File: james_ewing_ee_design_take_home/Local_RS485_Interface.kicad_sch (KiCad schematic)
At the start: 45 parts, among them J1 USB_B_Micro, J3 RJ45, J5 Conn_Coaxial, SW1 RST, SW2 RST, SW3 RST, U1 ESP8266EX, U1 SN65176BDR, U2 MCP2200-E-SS, U5 M95M02-DR, Y1 Resonator, Y2 TSX-3225

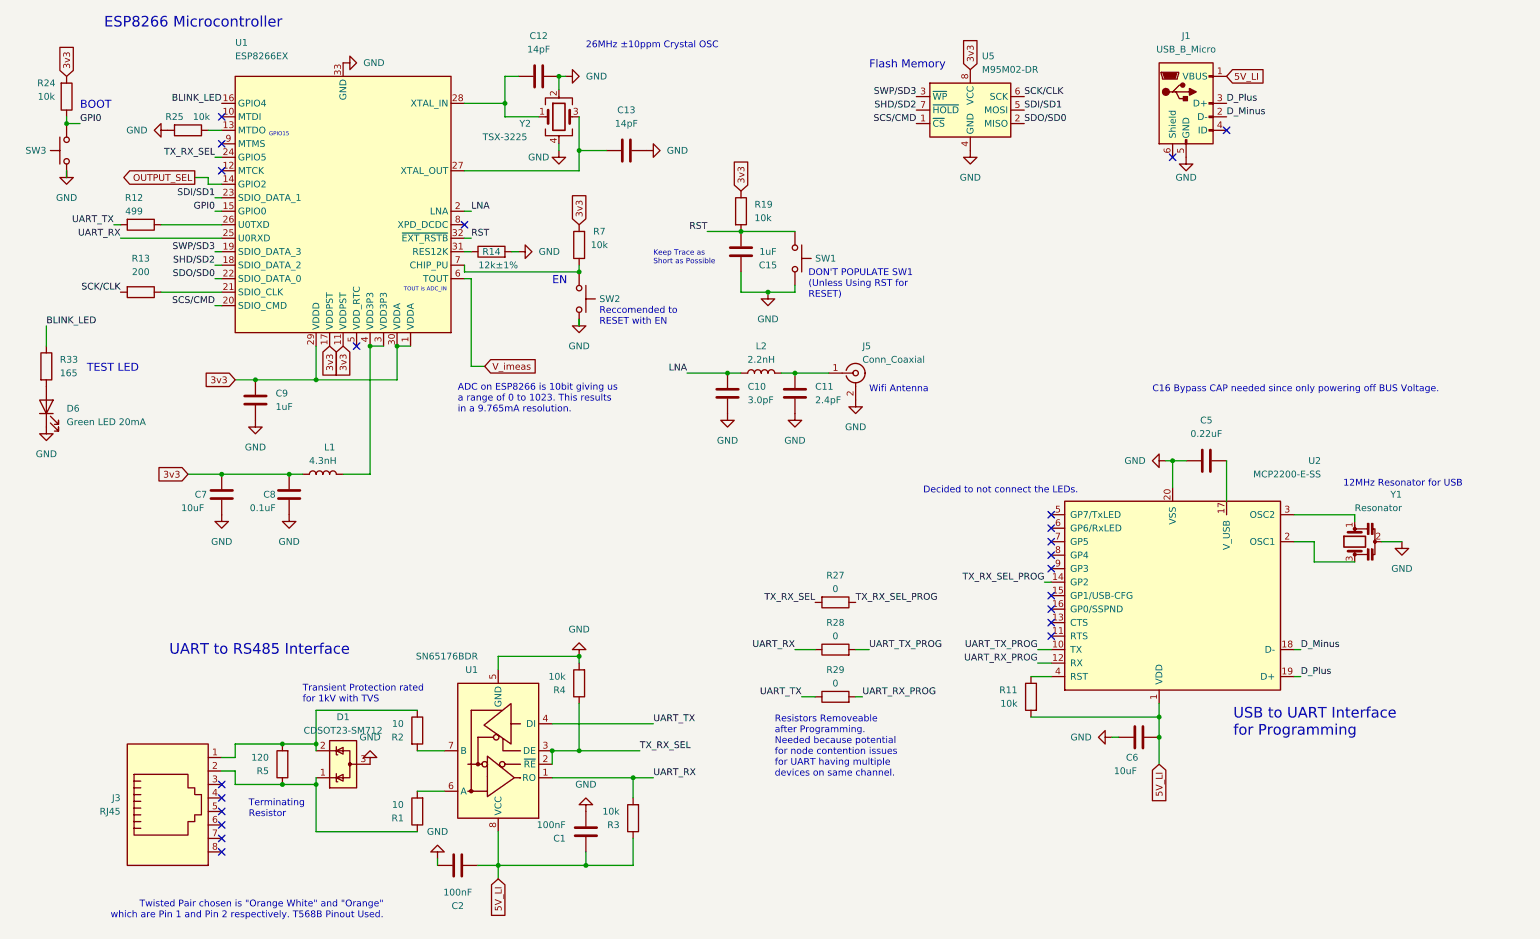
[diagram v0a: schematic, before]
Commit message: Updated Documentation
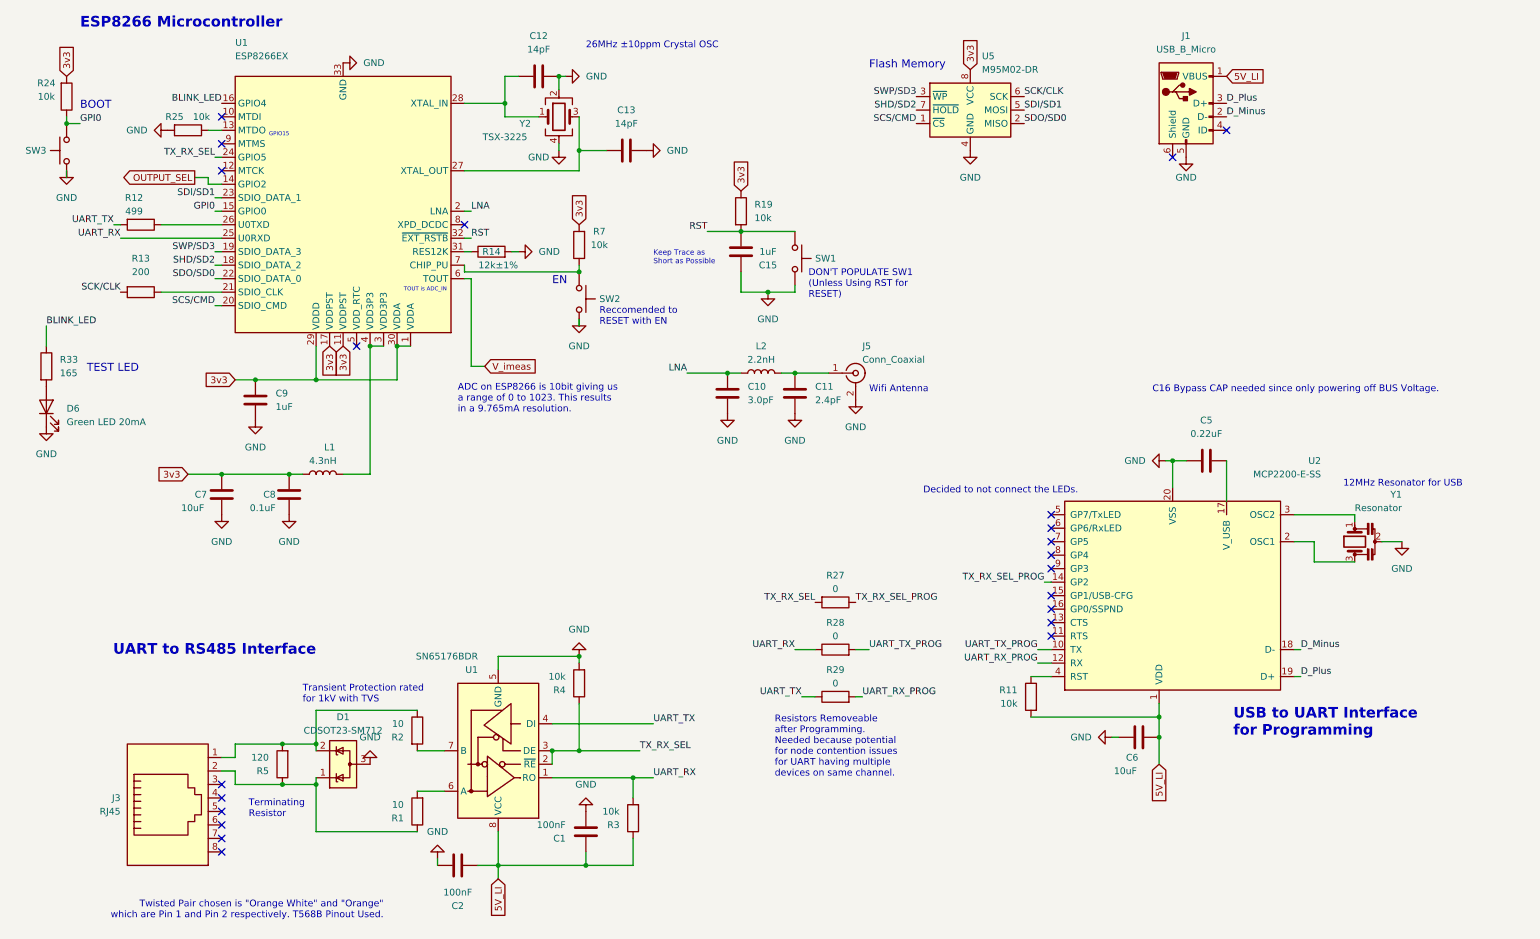
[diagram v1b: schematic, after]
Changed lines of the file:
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@@
   )
   (text "USB to UART Interface\nfor Programming" (at 240.03 153.67 0)
-    (effects (font (size 2 2)) (justify left bottom))
+    (effects (font (size 2 2) (thickness 0.4) bold) (justify left bottom))
   )
   (text "EN" (at 111.76 68.58 0)
@@
     (effects (font (size 1.27 1.27)) (justify left bottom))
   )
-  (text "UART to RS485 Interface" (at 73.66 138.43 0)
-    (effects (font (size 2 2)) (justify right bottom))
+  (text "UART to RS485 Interface" (at 67.31 138.43 0)
+    (effects (font (size 2 2) (thickness 0.4) bold) (justify right bottom))
   )
   (text "TEST LED" (at 24.13 85.09 0)
@@
   )
   (text "ESP8266 Microcontroller" (at 60.96 20.32 0)
-    (effects (font (size 2 2)) (justify right bottom))
+    (effects (font (size 2 2) (thickness 0.4) bold) (justify right bottom))
   )
   (text "Flash Memory" (at 171.45 27.94 0)
